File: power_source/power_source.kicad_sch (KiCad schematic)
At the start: 21 parts, among them J1 Traf secondary, J2 Traf Primary, J3 Input 230V AC, J4 Power, J5 5V DC, J6 12V DC, K1 SANYOU_SRD_Form_C, K2 SANYOU_SRD_Form_C, K3 SANYOU_SRD_Form_C, Q1 BC337, Q2 BC337, Q3 BC337, U1 ESP32-C3-DevKitM-1

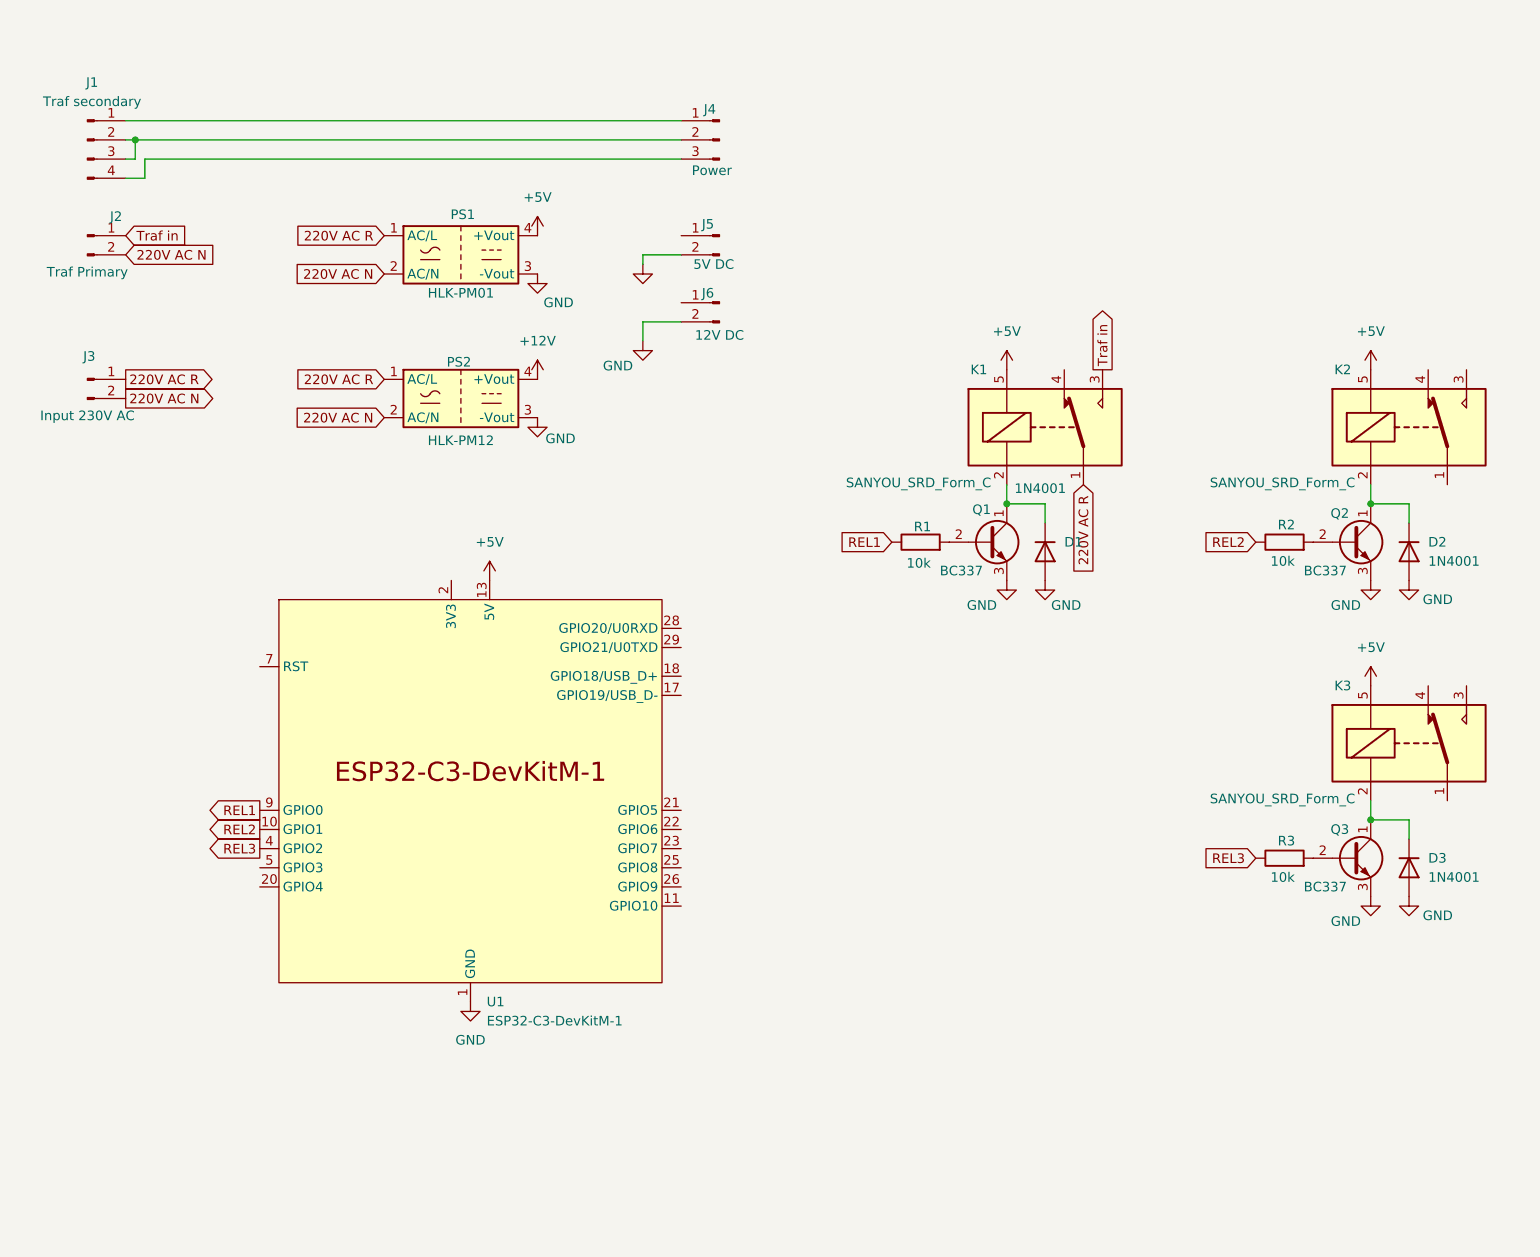
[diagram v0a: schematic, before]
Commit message: Wip
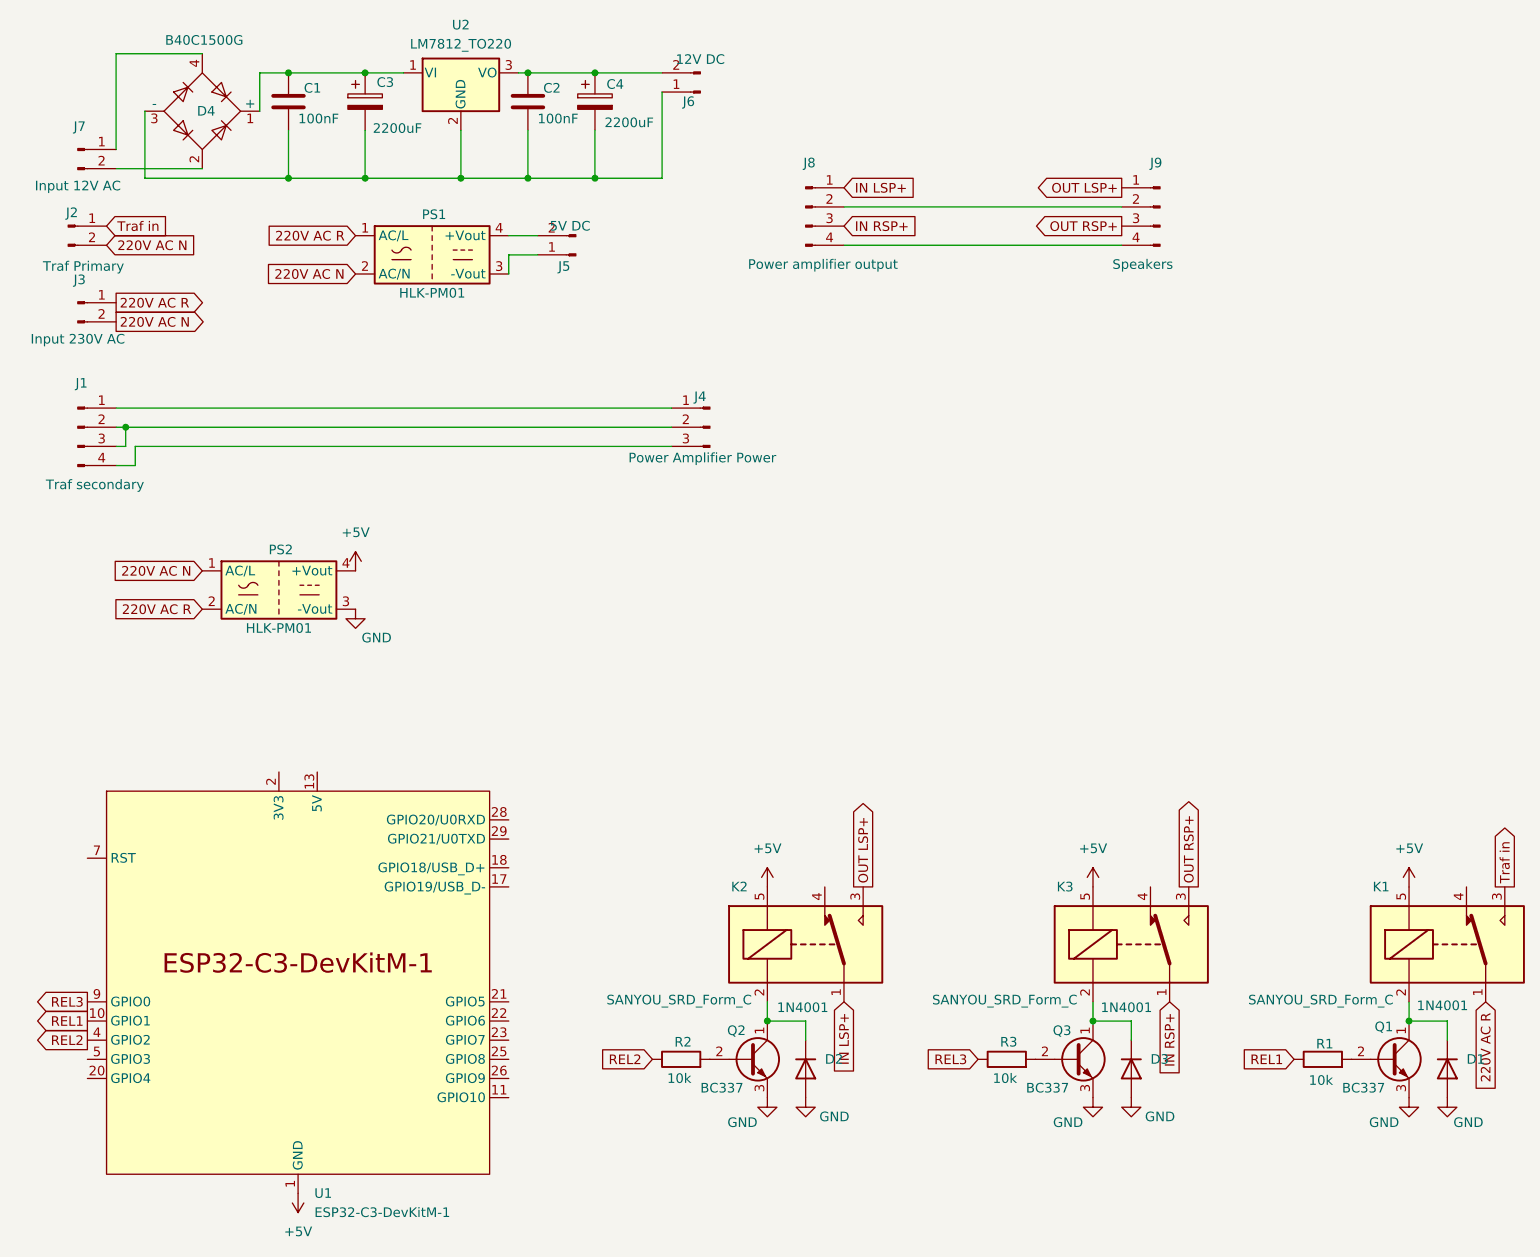
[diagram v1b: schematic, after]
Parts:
- removed PS2: HLK-PM12, Converter_ACDC:Converter_ACDC_Hi-Link_HLK-PMxx, symbol Converter_ACDC:HLK-PM12
- added C1, C2: 100nF, Capacitor_THT:C_Disc_D10.0mm_W2.5mm_P5.00mm, symbol Device:C
- added C3, C4: 2200uF, Capacitor_THT:CP_Radial_D18.0mm_P7.50mm, symbol Device:C_Polarized
- added D4: B40C1500G, Diode_THT:Diode_Bridge_Round_D9.8mm, symbol Diode_Bridge:B40C1500G
- added J7: Input 12V AC, Connector_Wire:SolderWire-0.5sqmm_1x02_P4.8mm_D0.9mm_OD2.3mm, symbol Connector:Conn_01x02_Pin
- added J8: Power amplifier output, Connector_Wire:SolderWire-0.5sqmm_1x04_P4.8mm_D0.9mm_OD2.3mm, symbol Connector:Conn_01x04_Pin
- added J9: Speakers, Connector_Wire:SolderWire-0.5sqmm_1x04_P4.8mm_D0.9mm_OD2.3mm, symbol Connector:Conn_01x04_Pin
- added PS2: HLK-PM01, Converter_ACDC:Converter_ACDC_Hi-Link_HLK-PMxx, symbol Converter_ACDC:HLK-PM01
- added U2: LM7812_TO220, Package_TO_SOT_THT:TO-220-3_Vertical, symbol Regulator_Linear:LM7812_TO220
- J1: footprint Connector_Wire:SolderWire-0.5sqmm_1x04_P4.6mm_D0.9mm_OD2.1mm -> Connector_Wire:SolderWire-0.5sqmm_1x04_P4.8mm_D0.9mm_OD2.3mm
- J2: footprint Connector_Wire:SolderWire-0.5sqmm_1x02_P4.6mm_D0.9mm_OD2.1mm -> Connector_Wire:SolderWire-0.75sqmm_1x02_P4.8mm_D1.25mm_OD2.3mm
- J3: footprint Connector_Wire:SolderWire-0.5sqmm_1x02_P4.6mm_D0.9mm_OD2.1mm -> Connector_Wire:SolderWire-0.5sqmm_1x02_P4.8mm_D0.9mm_OD2.3mm
- J4: value Power -> Power Amplifier Power
- J5, J6: footprint Connector_Wire:SolderWire-0.5sqmm_1x02_P4.6mm_D0.9mm_OD2.1mm -> Connector_JST:JST_XH_B2B-XH-A_1x02_P2.50mm_Vertical
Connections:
- net +5V: now also U1.1 (GND), U1.12 (GND), U1.15 (GND), U1.16 (GND), U1.19 (GND), U1.24 (GND), U1.27 (GND), U1.30 (GND), U1.6 (GND), U1.8 (GND), PS2.4 (+Vout); no longer PS1.4 (+Vout), U1.13 (5V), U1.14 (5V)
- net 220V AC N: now also PS2.1 (AC/L)
- net 220V AC R: now also PS2.2 (AC/N)
- net GND: now also PS2.3 (-Vout); no longer J5.2 (Pin_2), J6.2 (Pin_2), PS1.3 (-Vout), U1.1 (GND), U1.12 (GND), U1.15 (GND), U1.16 (GND), U1.19 (GND), U1.24 (GND), U1.27 (GND), U1.30 (GND), U1.6 (GND), U1.8 (GND)
- net REL1: now also U1.10 (GPIO1); no longer U1.9 (GPIO0)
- net REL2: now also U1.4 (GPIO2); no longer U1.10 (GPIO1)
- net REL3: now also U1.9 (GPIO0); no longer U1.4 (GPIO2)
- net at J6.1 (Pin_1): now also C1.2, C2.2, C3.2, C4.2, D4.3 (-), U2.2 (GND)
- net at J5.1 (Pin_1): now also PS1.3 (-Vout)
- net IN RSP+: now reaches K3.1
- net IN RSP+: now also J8.3 (Pin_3)
- net OUT RSP+: now reaches K3.3
- net OUT RSP+: now also J9.3 (Pin_3)
- net IN LSP+: now reaches K2.1
- net IN LSP+: now also J8.1 (Pin_1)
- net OUT LSP+: now reaches K2.3
- net OUT LSP+: now also J9.1 (Pin_1)
- new net: C2.1, C4.1, J6.2 (Pin_2), U2.3 (VO)
- new net: J8.2 (Pin_2), J9.2 (Pin_2)
- new net: J8.4 (Pin_4), J9.4 (Pin_4)
- new net: C1.1, C3.1, D4.1 (+), U2.1 (VI)
- new net: J5.2 (Pin_2), PS1.4 (+Vout)
- new net: D4.4, J7.1 (Pin_1)
- new net: D4.2, J7.2 (Pin_2)
- new net 5V: U1.13 (5V), U1.14 (5V)
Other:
- moved on the sheet: D1, D2, D3, J1, J2, J3, J4, J5, J6, K1, K2, K3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
